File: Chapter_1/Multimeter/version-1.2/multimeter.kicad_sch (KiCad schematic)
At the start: 67 parts, among them J1 Screw_Terminal_01x02, J2 Conn_01x02_Socket, J3 Screw_Terminal_01x02, Q1 IRLZ44N, Q17 BC547, Q18 BC547, Q19 BC547, Q20 BC547, Q22 BC547, Q23 BC547, Q24 BC547, Q25 BC547, Q26 BC547, Q27 BC547, Q28 BC547, Q29 BC547, Q30 BC547, Q31 BC547, Q32 BC547, Q33 IRLZ44N, Q34 IRLZ44N, SW1 SW_DPST_x2, SW2 SW_DPST_x2, SW3 SW_DPST_x2

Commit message: pcb adjusted size
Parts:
- R1, R10, R11, R12, R13, R14, R15, R16, R17, R18, R19, R2, R20, R21, R22, R23, R24, R25, R26, R27, R28, R29, R3, R30, R31, R32, R33, R4, R5, R6, R7, R8, R9: footprint Resistor_THT:R_Axial_DIN0309_L9.0mm_D3.2mm_P12.70mm_Horizontal -> Resistor_THT:R_Axial_DIN0309_L9.0mm_D3.2mm_P2.54mm_Vertical
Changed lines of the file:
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@@
 			)
 		)
-		(property "Footprint" "Resistor_THT:R_Axial_DIN0309_L9.0mm_D3.2mm_P12.70mm_Horizontal"
+		(property "Footprint" "Resistor_THT:R_Axial_DIN0309_L9.0mm_D3.2mm_P2.54mm_Vertical"
 			(at 179.07 32.512 90)
 			(effects
@@
 			)
 		)
-		(property "Footprint" "Resistor_THT:R_Axial_DIN0309_L9.0mm_D3.2mm_P12.70mm_Horizontal"
+		(property "Footprint" "Resistor_THT:R_Axial_DIN0309_L9.0mm_D3.2mm_P2.54mm_Vertical"
 			(at 82.55 55.372 90)
 			(effects
@@
 			)
 		)
-		(property "Footprint" "Resistor_THT:R_Axial_DIN0309_L9.0mm_D3.2mm_P12.70mm_Horizontal"
+		(property "Footprint" "Resistor_THT:R_Axial_DIN0309_L9.0mm_D3.2mm_P2.54mm_Vertical"
 			(at 78.74 109.728 90)
 			(effects
@@
 			)
 		)
-		(property "Footprint" "Resistor_THT:R_Axial_DIN0309_L9.0mm_D3.2mm_P12.70mm_Horizontal"
+		(property "Footprint" "Resistor_THT:R_Axial_DIN0309_L9.0mm_D3.2mm_P2.54mm_Vertical"
 			(at 160.02 105.918 90)
 			(effects
@@
 			)
 		)
-		(property "Footprint" "Resistor_THT:R_Axial_DIN0309_L9.0mm_D3.2mm_P12.70mm_Horizontal"
+		(property "Footprint" "Resistor_THT:R_Axial_DIN0309_L9.0mm_D3.2mm_P2.54mm_Vertical"
 			(at 151.13 166.878 90)
 			(effects
@@
 			)
 		)
-		(property "Footprint" "Resistor_THT:R_Axial_DIN0309_L9.0mm_D3.2mm_P12.70mm_Horizontal"
+		(property "Footprint" "Resistor_THT:R_Axial_DIN0309_L9.0mm_D3.2mm_P2.54mm_Vertical"
 			(at 77.47 64.008 90)
 			(effects
@@
 			)
 		)
-		(property "Footprint" "Resistor_THT:R_Axial_DIN0309_L9.0mm_D3.2mm_P12.70mm_Horizontal"
+		(property "Footprint" "Resistor_THT:R_Axial_DIN0309_L9.0mm_D3.2mm_P2.54mm_Vertical"
 			(at 242.57 61.468 90)
 			(effects
@@
 			)
 		)
-		(property "Footprint" "Resistor_THT:R_Axial_DIN0309_L9.0mm_D3.2mm_P12.70mm_Horizontal"
+		(property "Footprint" "Resistor_THT:R_Axial_DIN0309_L9.0mm_D3.2mm_P2.54mm_Vertical"
 			(at 66.04 81.788 90)
 			(effects
@@
 			)
 		)
-		(property "Footprint" "Resistor_THT:R_Axial_DIN0309_L9.0mm_D3.2mm_P12.70mm_Horizontal"
+		(property "Footprint" "Resistor_THT:R_Axial_DIN0309_L9.0mm_D3.2mm_P2.54mm_Vertical"
 			(at 265.938 78.74 90)
 			(effects
@@
 			)
 		)
-		(property "Footprint" "Resistor_THT:R_Axial_DIN0309_L9.0mm_D3.2mm_P12.70mm_Horizontal"
+		(property "Footprint" "Resistor_THT:R_Axial_DIN0309_L9.0mm_D3.2mm_P2.54mm_Vertical"
 			(at 114.3 51.308 90)
 			(effects
@@
 			)
 		)
-		(property "Footprint" "Resistor_THT:R_Axial_DIN0309_L9.0mm_D3.2mm_P12.70mm_Horizontal"
+		(property "Footprint" "Resistor_THT:R_Axial_DIN0309_L9.0mm_D3.2mm_P2.54mm_Vertical"
 			(at 67.31 127.508 90)
 			(effects
@@
 			)
 		)
-		(property "Footprint" "Resistor_THT:R_Axial_DIN0309_L9.0mm_D3.2mm_P12.70mm_Horizontal"
+		(property "Footprint" "Resistor_THT:R_Axial_DIN0309_L9.0mm_D3.2mm_P2.54mm_Vertical"
 			(at 261.62 90.678 90)
 			(effects
@@
 			)
 		)
-		(property "Footprint" "Resistor_THT:R_Axial_DIN0309_L9.0mm_D3.2mm_P12.70mm_Horizontal"
+		(property "Footprint" "Resistor_THT:R_Axial_DIN0309_L9.0mm_D3.2mm_P2.54mm_Vertical"
 			(at 251.46 80.518 90)
 			(effects
@@
 			)
 		)
-		(property "Footprint" "Resistor_THT:R_Axial_DIN0309_L9.0mm_D3.2mm_P12.70mm_Horizontal"
+		(property "Footprint" "Resistor_THT:R_Axial_DIN0309_L9.0mm_D3.2mm_P2.54mm_Vertical"
 			(at 55.88 47.498 90)
 			(effects
@@
 			)
 		)
-		(property "Footprint" "Resistor_THT:R_Axial_DIN0309_L9.0mm_D3.2mm_P12.70mm_Horizontal"
+		(property "Footprint" "Resistor_THT:R_Axial_DIN0309_L9.0mm_D3.2mm_P2.54mm_Vertical"
 			(at 173.99 41.148 90)
 			(effects
@@
 			)
 		)
-		(property "Footprint" "Resistor_THT:R_Axial_DIN0309_L9.0mm_D3.2mm_P12.70mm_Horizontal"
+		(property "Footprint" "Resistor_THT:R_Axial_DIN0309_L9.0mm_D3.2mm_P2.54mm_Vertical"
 			(at 166.37 40.132 90)
 			(effects
@@
 			)
 		)
-		(property "Footprint" "Resistor_THT:R_Axial_DIN0309_L9.0mm_D3.2mm_P12.70mm_Horizontal"
+		(property "Footprint" "Resistor_THT:R_Axial_DIN0309_L9.0mm_D3.2mm_P2.54mm_Vertical"
 			(at 238.76 72.898 90)
 			(effects
@@
 			)
 		)
-		(property "Footprint" "Resistor_THT:R_Axial_DIN0309_L9.0mm_D3.2mm_P12.70mm_Horizontal"
+		(property "Footprint" "Resistor_THT:R_Axial_DIN0309_L9.0mm_D3.2mm_P2.54mm_Vertical"
 			(at 196.85 32.258 90)
 			(effects
@@
 			)
 		)
-		(property "Footprint" "Resistor_THT:R_Axial_DIN0309_L9.0mm_D3.2mm_P12.70mm_Horizontal"
+		(property "Footprint" "Resistor_THT:R_Axial_DIN0309_L9.0mm_D3.2mm_P2.54mm_Vertical"
 			(at 66.04 71.628 90)
 			(effects
@@
 			)
 		)
-		(property "Footprint" "Resistor_THT:R_Axial_DIN0309_L9.0mm_D3.2mm_P12.70mm_Horizontal"
+		(property "Footprint" "Resistor_THT:R_Axial_DIN0309_L9.0mm_D3.2mm_P2.54mm_Vertical"
 			(at 167.64 150.622 90)
 			(effects
@@
 			)
 		)
-		(property "Footprint" "Resistor_THT:R_Axial_DIN0309_L9.0mm_D3.2mm_P12.70mm_Horizontal"
+		(property "Footprint" "Resistor_THT:R_Axial_DIN0309_L9.0mm_D3.2mm_P2.54mm_Vertical"
 			(at 71.12 108.712 90)
 			(effects
@@
 			)
 		)
-		(property "Footprint" "Resistor_THT:R_Axial_DIN0309_L9.0mm_D3.2mm_P12.70mm_Horizontal"
+		(property "Footprint" "Resistor_THT:R_Axial_DIN0309_L9.0mm_D3.2mm_P2.54mm_Vertical"
 			(at 148.59 113.538 90)
 			(effects
@@
 			)
 		)
-		(property "Footprint" "Resistor_THT:R_Axial_DIN0309_L9.0mm_D3.2mm_P12.70mm_Horizontal"
+		(property "Footprint" "Resistor_THT:R_Axial_DIN0309_L9.0mm_D3.2mm_P2.54mm_Vertical"
 			(at 162.56 58.928 90)
 			(effects
@@
 			)
 		)
-		(property "Footprint" "Resistor_THT:R_Axial_DIN0309_L9.0mm_D3.2mm_P12.70mm_Horizontal"
+		(property "Footprint" "Resistor_THT:R_Axial_DIN0309_L9.0mm_D3.2mm_P2.54mm_Vertical"
 			(at 83.82 101.092 90)
 			(effects
@@
 			)
 		)
-		(property "Footprint" "Resistor_THT:R_Axial_DIN0309_L9.0mm_D3.2mm_P12.70mm_Horizontal"
+		(property "Footprint" "Resistor_THT:R_Axial_DIN0309_L9.0mm_D3.2mm_P2.54mm_Vertical"
 			(at 69.85 62.992 90)
 			(effects
@@
 			)
 		)
-		(property "Footprint" "Resistor_THT:R_Axial_DIN0309_L9.0mm_D3.2mm_P12.70mm_Horizontal"
+		(property "Footprint" "Resistor_THT:R_Axial_DIN0309_L9.0mm_D3.2mm_P2.54mm_Vertical"
 			(at 154.94 158.242 90)
 			(effects
@@
 			)
 		)
-		(property "Footprint" "Resistor_THT:R_Axial_DIN0309_L9.0mm_D3.2mm_P12.70mm_Horizontal"
+		(property "Footprint" "Resistor_THT:R_Axial_DIN0309_L9.0mm_D3.2mm_P2.54mm_Vertical"
 			(at 152.4 104.902 90)
 			(effects
@@
 			)
 		)
-		(property "Footprint" "Resistor_THT:R_Axial_DIN0309_L9.0mm_D3.2mm_P12.70mm_Horizontal"
+		(property "Footprint" "Resistor_THT:R_Axial_DIN0309_L9.0mm_D3.2mm_P2.54mm_Vertical"
 			(at 148.59 123.698 90)
 			(effects
@@
 			)
 		)
-		(property "Footprint" "Resistor_THT:R_Axial_DIN0309_L9.0mm_D3.2mm_P12.70mm_Horizontal"
+		(property "Footprint" "Resistor_THT:R_Axial_DIN0309_L9.0mm_D3.2mm_P2.54mm_Vertical"
 			(at 151.13 177.038 90)
 			(effects
@@
 			)
 		)
-		(property "Footprint" "Resistor_THT:R_Axial_DIN0309_L9.0mm_D3.2mm_P12.70mm_Horizontal"
+		(property "Footprint" "Resistor_THT:R_Axial_DIN0309_L9.0mm_D3.2mm_P2.54mm_Vertical"
 			(at 162.56 48.768 90)
 			(effects
@@
 			)
 		)
-		(property "Footprint" "Resistor_THT:R_Axial_DIN0309_L9.0mm_D3.2mm_P12.70mm_Horizontal"
+		(property "Footprint" "Resistor_THT:R_Axial_DIN0309_L9.0mm_D3.2mm_P2.54mm_Vertical"
 			(at 165.1 97.282 90)
 			(effects
@@
 			)
 		)
-		(property "Footprint" "Resistor_THT:R_Axial_DIN0309_L9.0mm_D3.2mm_P12.70mm_Horizontal"
+		(property "Footprint" "Resistor_THT:R_Axial_DIN0309_L9.0mm_D3.2mm_P2.54mm_Vertical"
 			(at 162.56 159.258 90)
 			(effects
@@
 			)
 		)
-		(property "Footprint" "Resistor_THT:R_Axial_DIN0309_L9.0mm_D3.2mm_P12.70mm_Horizontal"
+		(property "Footprint" "Resistor_THT:R_Axial_DIN0309_L9.0mm_D3.2mm_P2.54mm_Vertical"
 			(at 67.31 117.348 90)
 			(effects

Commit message: .
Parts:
- Q17, Q18, Q19, Q20, Q22, Q23, Q24, Q25, Q26, Q27, Q28, Q29, Q30, Q31, Q32: footprint Package_TO_SOT_THT:TO-92_Inline -> Package_TO_SOT_THT:TO-92L_Inline_Wide
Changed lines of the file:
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@@
 			)
 		)
-		(property "Footprint" "Package_TO_SOT_THT:TO-92_Inline"
+		(property "Footprint" "Package_TO_SOT_THT:TO-92L_Inline_Wide"
 			(at 81.28 117.475 0)
 			(effects
@@
 			)
 		)
-		(property "Footprint" "Package_TO_SOT_THT:TO-92_Inline"
+		(property "Footprint" "Package_TO_SOT_THT:TO-92L_Inline_Wide"
 			(at 80.01 81.915 0)
 			(effects
@@
 			)
 		)
-		(property "Footprint" "Package_TO_SOT_THT:TO-92_Inline"
+		(property "Footprint" "Package_TO_SOT_THT:TO-92L_Inline_Wide"
 			(at 92.71 109.855 0)
 			(effects
@@
 			)
 		)
-		(property "Footprint" "Package_TO_SOT_THT:TO-92_Inline"
+		(property "Footprint" "Package_TO_SOT_THT:TO-92L_Inline_Wide"
 			(at 187.96 41.275 0)
 			(effects
@@
 			)
 		)
-		(property "Footprint" "Package_TO_SOT_THT:TO-92_Inline"
+		(property "Footprint" "Package_TO_SOT_THT:TO-92L_Inline_Wide"
 			(at 165.1 177.165 0)
 			(effects
@@
 			)
 		)
-		(property "Footprint" "Package_TO_SOT_THT:TO-92_Inline"
+		(property "Footprint" "Package_TO_SOT_THT:TO-92L_Inline_Wide"
 			(at 80.01 71.755 0)
 			(effects
@@
 			)
 		)
-		(property "Footprint" "Package_TO_SOT_THT:TO-92_Inline"
+		(property "Footprint" "Package_TO_SOT_THT:TO-92L_Inline_Wide"
 			(at 165.1 167.005 0)
 			(effects
@@
 			)
 		)
-		(property "Footprint" "Package_TO_SOT_THT:TO-92_Inline"
+		(property "Footprint" "Package_TO_SOT_THT:TO-92L_Inline_Wide"
 			(at 81.28 127.635 0)
 			(effects
@@
 			)
 		)
-		(property "Footprint" "Package_TO_SOT_THT:TO-92_Inline"
+		(property "Footprint" "Package_TO_SOT_THT:TO-92L_Inline_Wide"
 			(at 162.56 113.665 0)
 			(effects
@@
 			)
 		)
-		(property "Footprint" "Package_TO_SOT_THT:TO-92_Inline"
+		(property "Footprint" "Package_TO_SOT_THT:TO-92L_Inline_Wide"
 			(at 176.53 48.895 0)
 			(effects
@@
 			)
 		)
-		(property "Footprint" "Package_TO_SOT_THT:TO-92_Inline"
+		(property "Footprint" "Package_TO_SOT_THT:TO-92L_Inline_Wide"
 			(at 173.99 106.045 0)
 			(effects
@@
 			)
 		)
-		(property "Footprint" "Package_TO_SOT_THT:TO-92_Inline"
+		(property "Footprint" "Package_TO_SOT_THT:TO-92L_Inline_Wide"
 			(at 176.53 159.385 0)
 			(effects
@@
 			)
 		)
-		(property "Footprint" "Package_TO_SOT_THT:TO-92_Inline"
+		(property "Footprint" "Package_TO_SOT_THT:TO-92L_Inline_Wide"
 			(at 176.53 59.055 0)
 			(effects
@@
 			)
 		)
-		(property "Footprint" "Package_TO_SOT_THT:TO-92_Inline"
+		(property "Footprint" "Package_TO_SOT_THT:TO-92L_Inline_Wide"
 			(at 91.44 64.135 0)
 			(effects
@@
 			)
 		)
-		(property "Footprint" "Package_TO_SOT_THT:TO-92_Inline"
+		(property "Footprint" "Package_TO_SOT_THT:TO-92L_Inline_Wide"
 			(at 162.56 123.825 0)
 			(effects

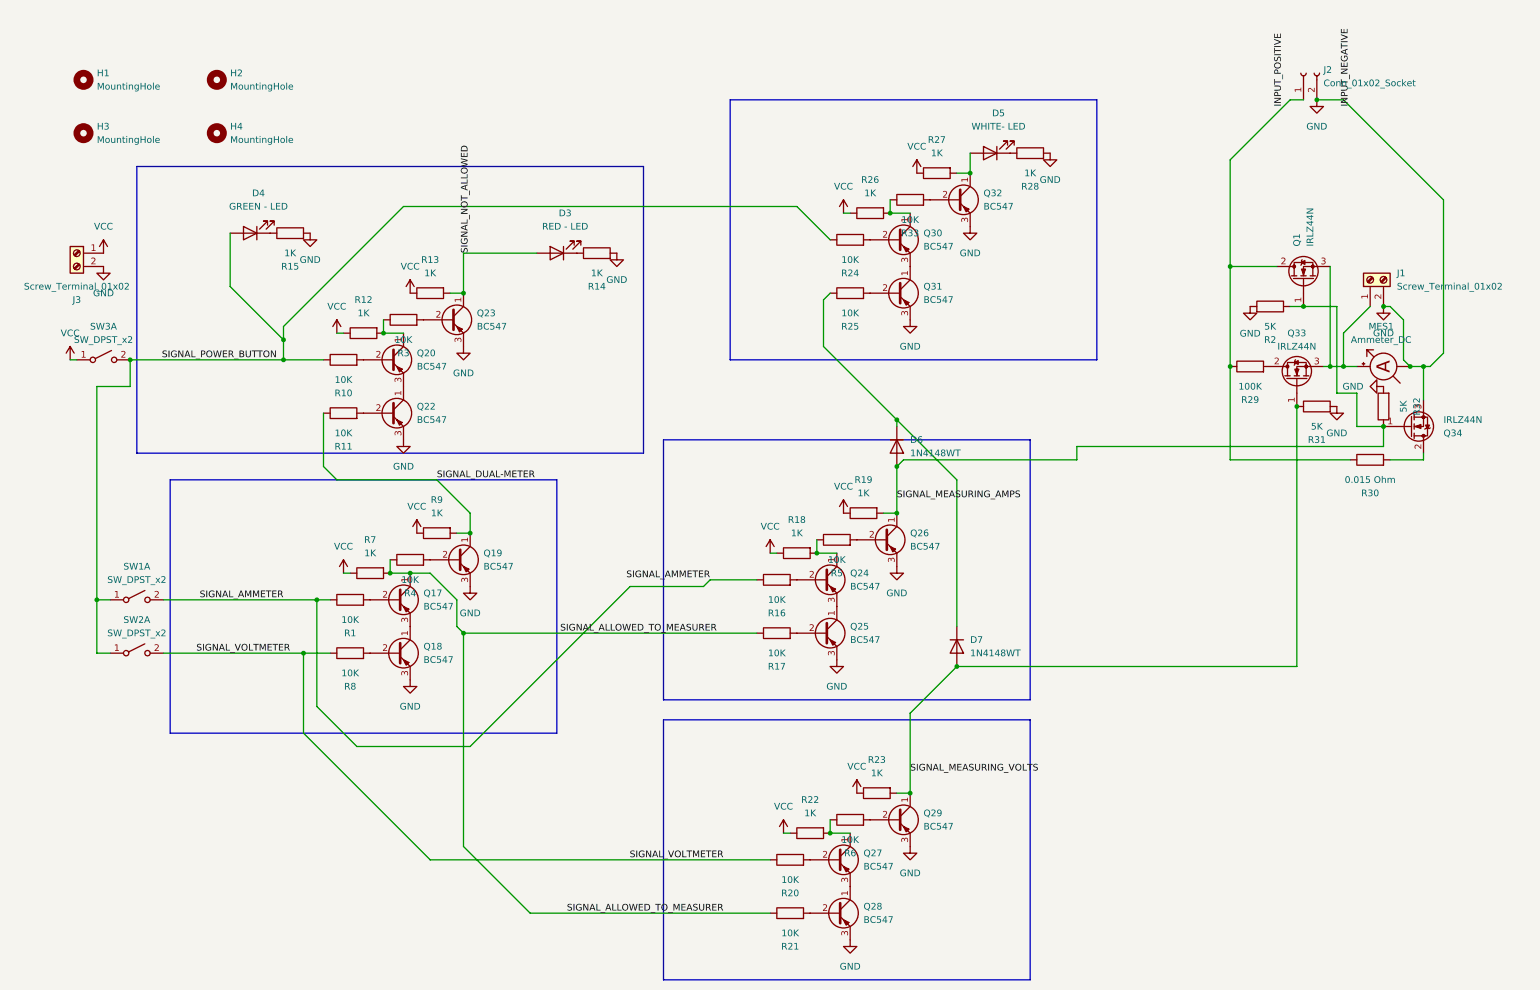
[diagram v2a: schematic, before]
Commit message: .
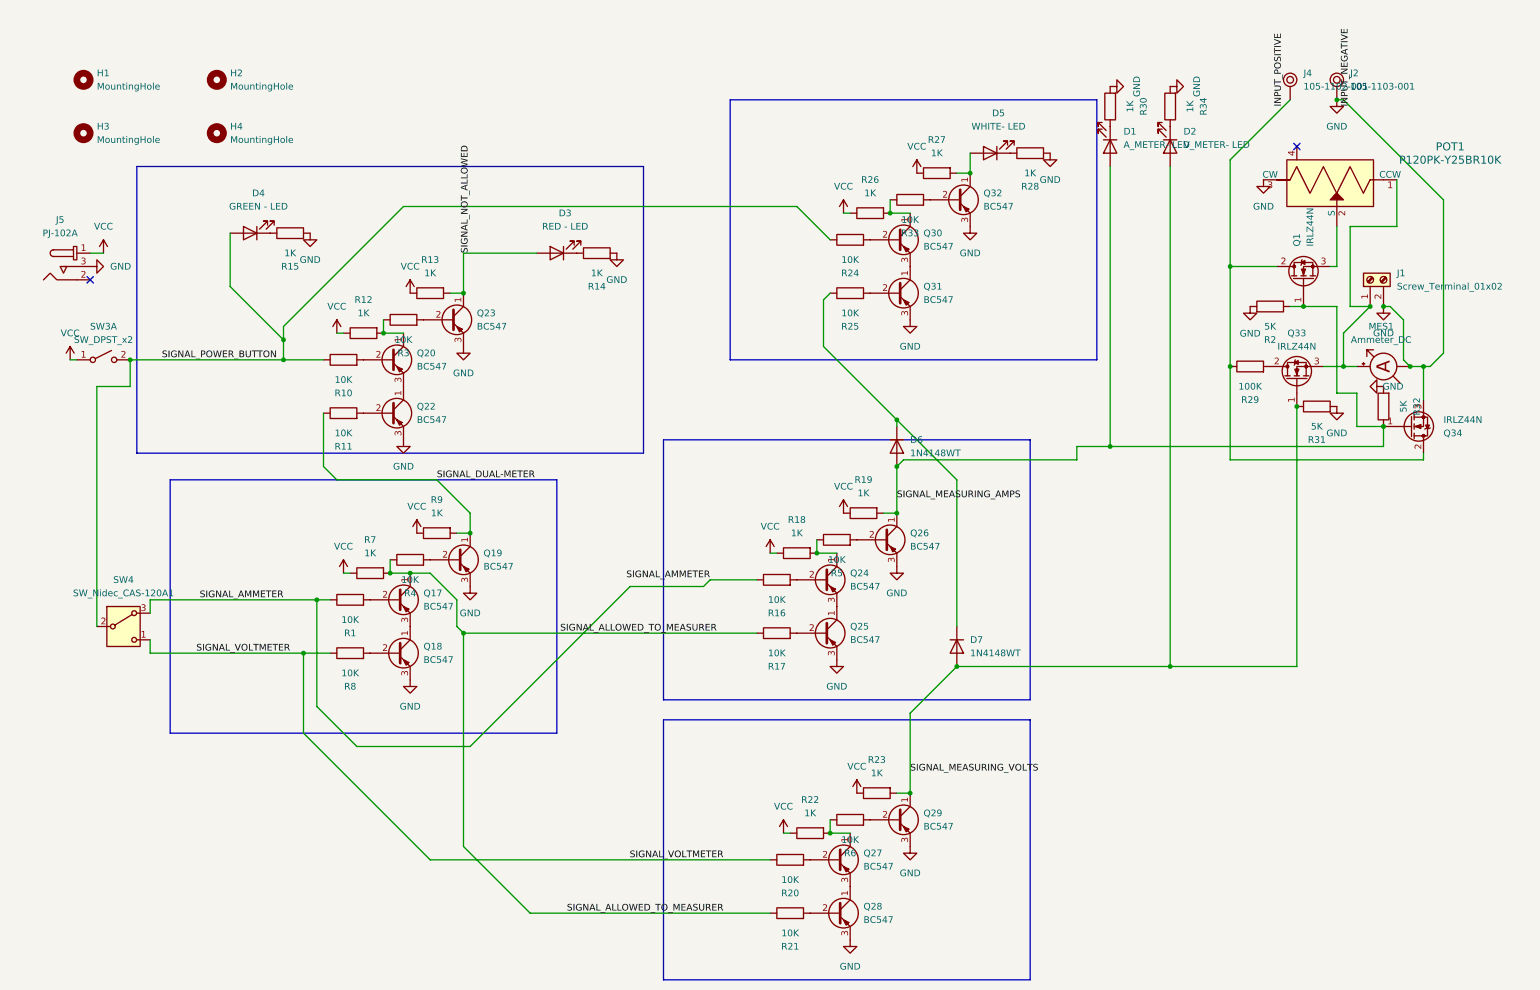
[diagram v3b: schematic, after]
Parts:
- removed J2: Conn_01x02_Socket, TerminalBlock:TerminalBlock_MaiXu_MX126-5.0-02P_1x02_P5.00mm, symbol Connector:Conn_01x02_Socket
- removed J3: Screw_Terminal_01x02, TerminalBlock:TerminalBlock_MaiXu_MX126-5.0-02P_1x02_P5.00mm, symbol Connector:Screw_Terminal_01x02
- removed SW1, SW2: SW_DPST_x2, Button_Switch_THT:SW_DIP_SPSTx01_Piano_10.8x4.1mm_W7.62mm_P2.54mm, symbol Switch:SW_DPST_x2
- added D1: A_METER- LED, LED_THT:LED_D1.8mm_W3.3mm_H2.4mm, symbol Device:LED
- added D2: V_METER- LED, LED_THT:LED_D1.8mm_W3.3mm_H2.4mm, symbol Device:LED
- added J2: 105-1103-001, digikey-footprints:Test_Jack_Horiz, symbol dk_Banana-and-Tip-Connectors-Jacks-Plugs:105-1103-001
- added J4: 105-1102-001, digikey-footprints:Test_Jack_Horiz, symbol dk_Banana-and-Tip-Connectors-Jacks-Plugs:105-1102-001
- added J5: PJ-102A, digikey-footprints:Barrel_Jack_5.5mmODx2.1mmID_PJ-102A, symbol dk_Barrel-Power-Connectors:PJ-102A
- added POT1: P120PK-Y25BR10K, digikey-footprints:Potentiometer_P120PK-Y25BR10K, symbol dk_Rotary-Potentiometers-Rheostats:P120PK-Y25BR10K
- added R34: 1K, Resistor_THT:R_Axial_DIN0207_L6.3mm_D2.5mm_P10.16mm_Horizontal, symbol Device:R
- added SW4: SW_Nidec_CAS-120A1, digikey-footprints:Switch_Toggle_ATE1D-2M3-10-Z, symbol Switch:SW_Nidec_CAS-120A1
- Q17, Q18, Q19, Q20, Q22, Q23, Q24, Q25, Q26, Q27, Q28, Q29, Q30, Q31, Q32: footprint Package_TO_SOT_THT:TO-92L_Inline_Wide -> Package_TO_SOT_THT:TO-92_HandSolder
- R1, R10, R11, R12, R13, R14, R15, R16, R17, R18, R19, R2, R20, R21, R22, R23, R24, R25, R26, R27, R28, R29, R3, R31, R32, R33, R4, R5, R6, R7, R8, R9: footprint Resistor_THT:R_Axial_DIN0309_L9.0mm_D3.2mm_P2.54mm_Vertical -> Resistor_THT:R_Axial_DIN0207_L6.3mm_D2.5mm_P10.16mm_Horizontal
- R30: value 0.015 Ohm -> 1K; footprint Resistor_THT:R_Axial_DIN0309_L9.0mm_D3.2mm_P2.54mm_Vertical -> Resistor_THT:R_Axial_DIN0207_L6.3mm_D2.5mm_P10.16mm_Horizontal
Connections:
- net GND: now also R30.2, J2.1, J5.3, POT1.3 (CW), R34.2
- net INPUT_POSITIVE: now also Q34.2 (D), J4.1; no longer R30.1
- net SIGNAL_AMMETER: now also SW4.3 (A)
- net SIGNAL_MEASURING_AMPS: now also D1.2 (A)
- net SIGNAL_MEASURING_VOLTS: now also D2.2 (A)
- net SIGNAL_POWER_BUTTON: now also SW4.2 (B)
- net SIGNAL_VOLTMETER: now also SW4.1 (C)
- net VCC: now also J5.1
- net at J1.1 (Pin_1), MES1.2 (+), Q33.3 (S): now also POT1.1 (CCW); no longer Q1.3 (S)
- new net: D1.1 (K), R30.1
- new net: POT1.2 (S), Q1.3 (S)
- new net: D2.1 (K), R34.1
- no-connect marks 0 -> 2
